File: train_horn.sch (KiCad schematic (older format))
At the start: 46 parts

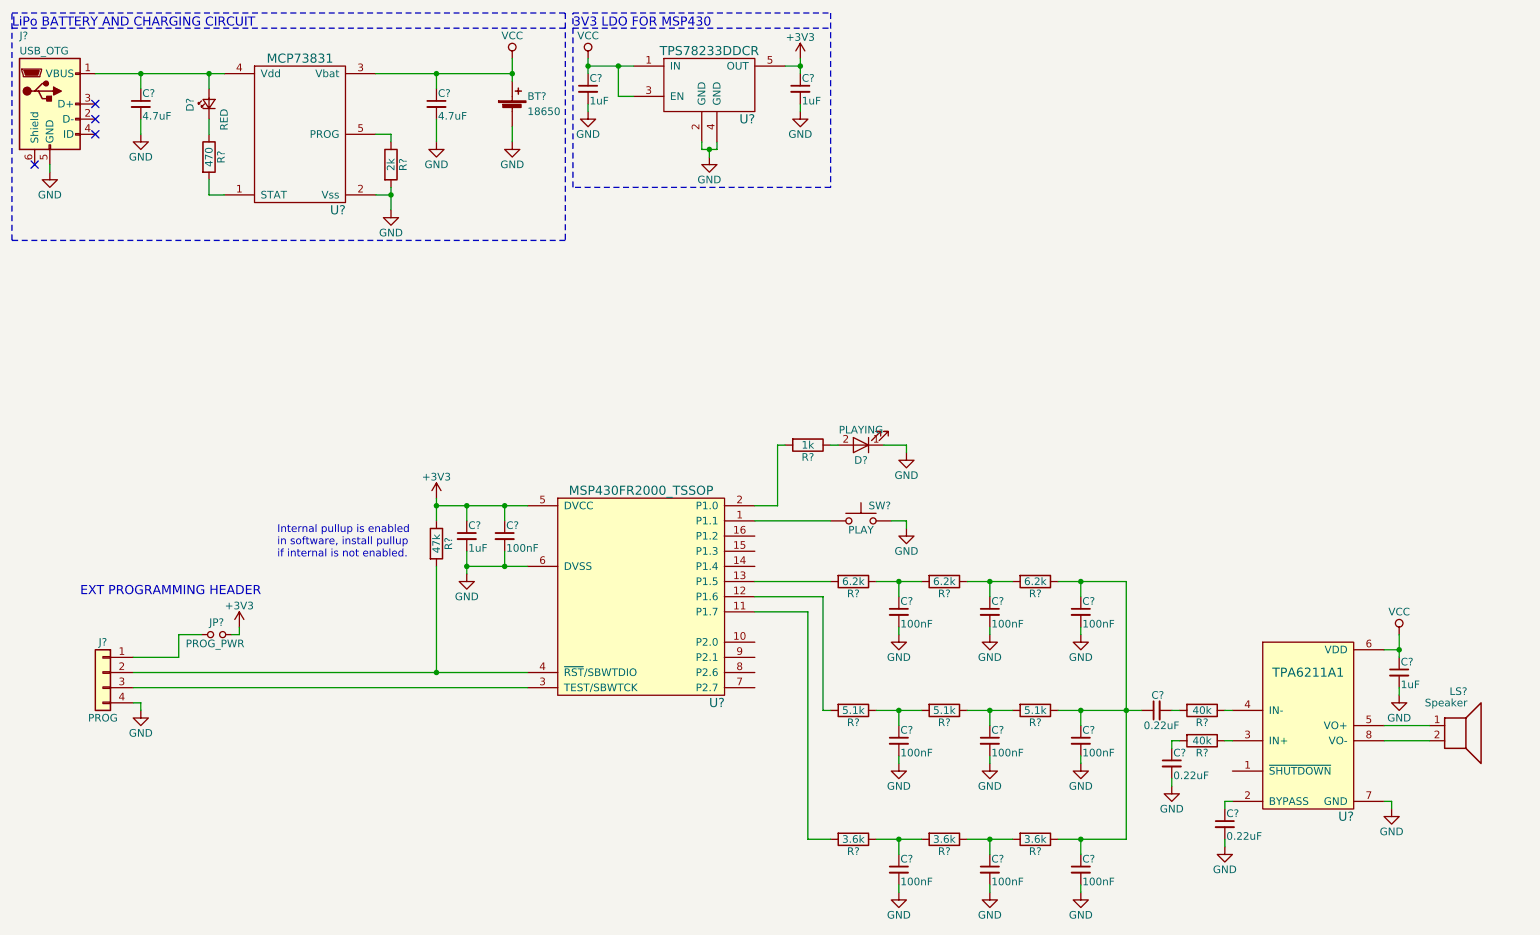
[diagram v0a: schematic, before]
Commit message: initial final schematic
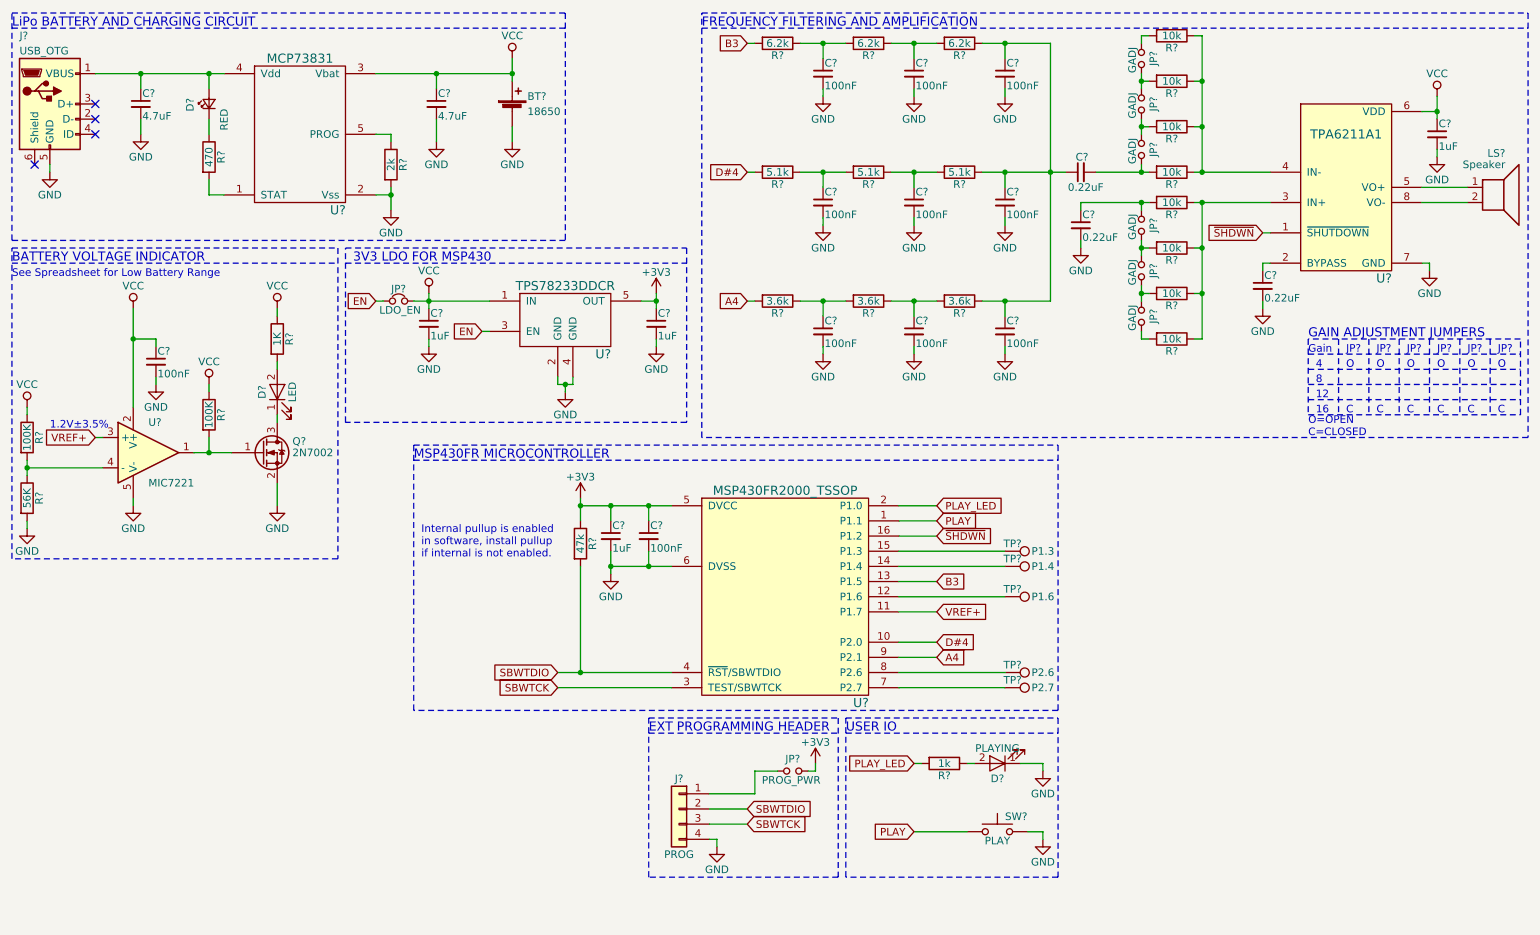
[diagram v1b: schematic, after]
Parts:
- removed R? (x2): 40k, symbol R
- added C?: 100nF, symbol C_Small
- added D?: LED, symbol LED
- added JP?: LDO_EN, symbol Jumper_NC_Small
- added JP? (x6): GADJ, symbol Jumper_NO_Small
- added Q?: 2N7002, TO_SOT_Packages_SMD:SOT-23, symbol 2N7002
- added R? (x2): 100K, symbol R
- added R?: 56K, symbol R
- added R?: 1K, symbol R
- added R? (x8): 10k, symbol R
- added TP?: P1.3, symbol Test_Point
- added TP?: P1.4, symbol Test_Point
- added TP?: P1.6, symbol Test_Point
- added TP?: P2.6, symbol Test_Point
- added TP?: P2.7, symbol Test_Point
- added U?: MIC7221, TO_SOT_Packages_SMD:SOT-23-5, symbol MCP6566R
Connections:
- net GND: now also C?.2, Q?.2 (S), R?.2, U?.5 (V-)
- net VCC: now also C?.1, JP?.2, R?.1, R?.1, R?.1, U?.2 (V+); no longer U?.3 (EN)
- net PLAY: now reaches SW?.1, U?.1 (P1.1)
- net D#4: now reaches U?.10 (P2.0)
- net D#4: now also R?.2
- net A4: now reaches R?.2
- net A4: now also U?.9 (P2.1); no longer U?.11 (P1.7)
- net at U?.12 (P1.6): now also TP?.1; no longer R?.2
- net B3: now reaches R?.2, U?.13 (P1.5)
- net at U?.14 (P1.4): now also TP?.1
- net at U?.15 (P1.3): now also TP?.1
- net ~SHDWN: now reaches U?.16 (P1.2)
- net ~SHDWN: now also U?.1 (~SHUTDOWN)
- net PLAY_LED: now reaches R?.2, U?.2 (P1.0)
- net SBWTCK: now reaches J?.3 (Pin_3), U?.3 (TEST/SBWTCK)
- net SBWTDIO: now reaches J?.2 (Pin_2), R?.2, U?.4 (~RST~/SBWTDIO)
- net at U?.7 (P2.7): now also TP?.1
- net at U?.8 (P2.6): now also TP?.1
- net at U?.3 (IN+): now also R?.1, R?.1, R?.1, R?.1
- net at U?.4 (IN-): now also R?.1, R?.1, R?.1, R?.1
- net at C?.2: now also JP?.2, R?.2
- net at C?.1: now also JP?.1, R?.2
- new net: R?.1, R?.2, U?.4 (-)
- new net: Q?.1 (G), R?.2, U?.1
- new net: D?.1 (K), Q?.3 (D)
- new net: D?.2 (A), R?.2
- new net: JP?.1, R?.2
- new net: JP?.1, JP?.2, R?.2 (x4)
- new net: JP?.2, R?.2
- new net EN: JP?.1, U?.3 (EN)
- new net VREF+: U?.11 (P1.7), U?.3 (+)
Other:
- note added: "1.2V±3.5%"
- note added: "12"
- note added: "16"
- note added: "4"
- note added: "8"
- note added: "BATTERY VOLTAGE INDICATOR"
- note added: "C"
- note added: "FREQUENCY FILTERING AND AMPLIFICATION"
- note added: "GAIN ADJUSTMENT JUMPERS"
- note added: "Gain"
- note added: "JP?"
- note added: "MSP430FR MICROCONTROLLER"
- note added: "O"
- note added: "O=OPEN\nC=CLOSED"
- note added: "See Spreadsheet for Low Battery Range"
- note added: "USER IO"
- moved on the sheet: C?, D?, J?, JP?, LS?, R?, SW?, U?
